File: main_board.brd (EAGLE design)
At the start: 123.2 x 81 mm, 46 parts, among them P1 ST-TF-003A, U1 STM32F407VGT6, U2 USBLC6-2, U3 MCP1700T-3302E, U4 LTC4054LES5-4.2#TRPBF, X1 MicroUSB-B

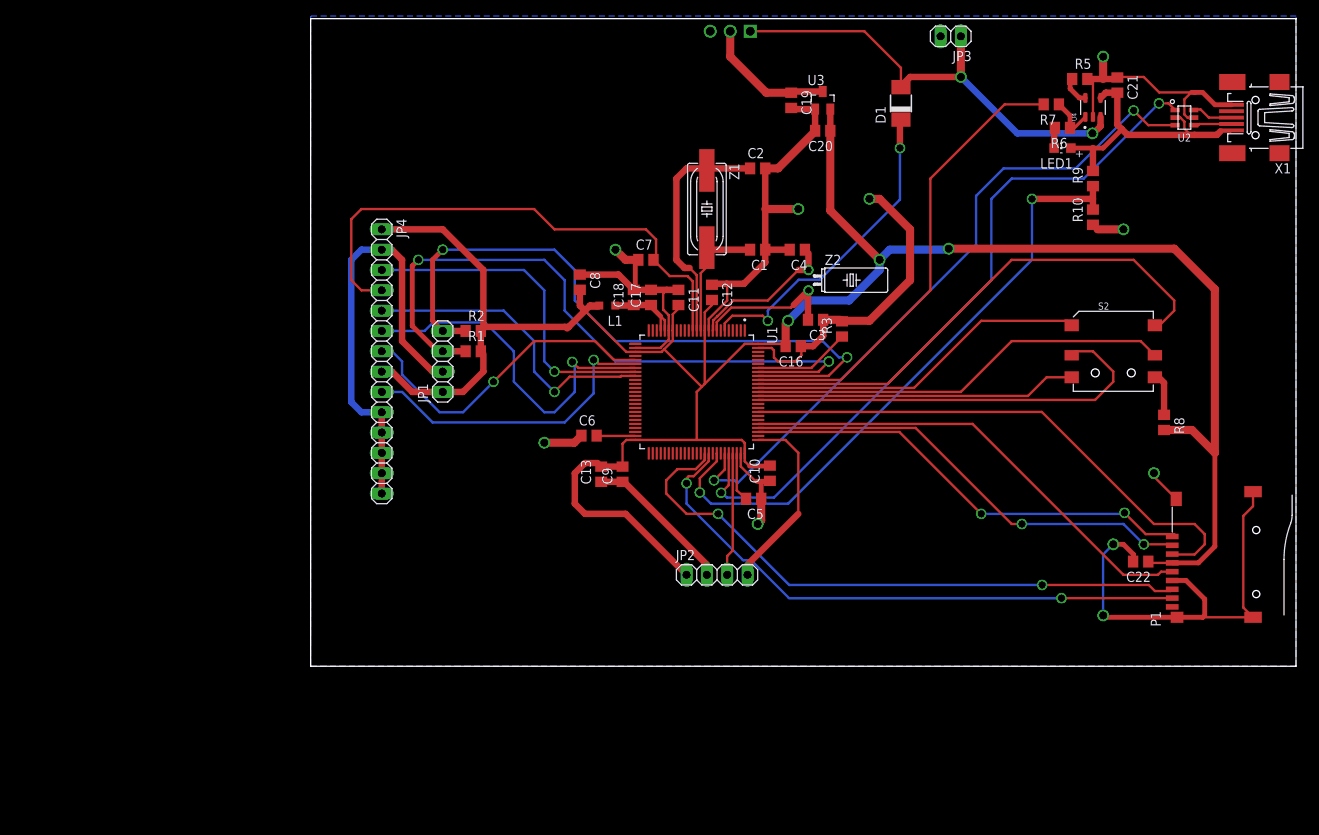
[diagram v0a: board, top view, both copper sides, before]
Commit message: pcb almost done
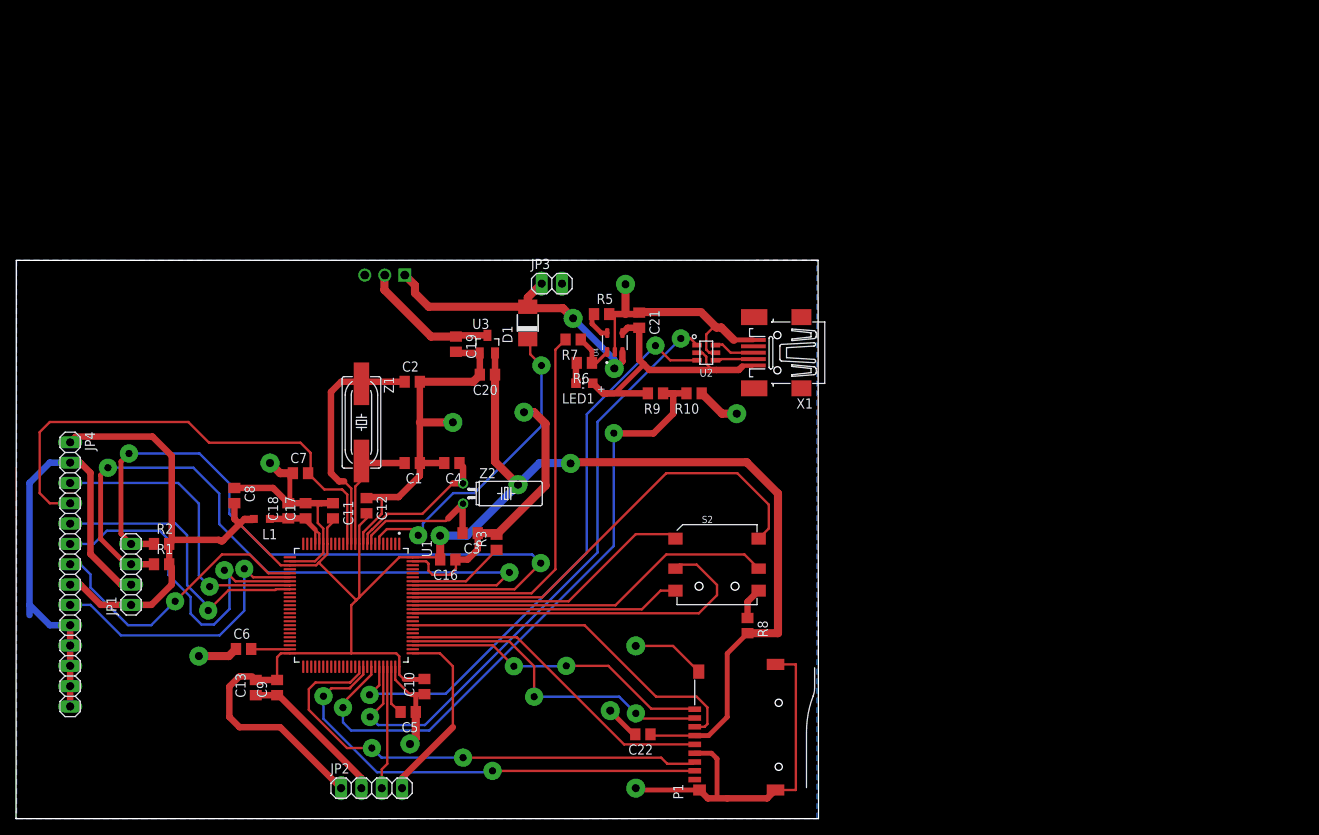
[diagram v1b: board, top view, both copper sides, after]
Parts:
- moved C21 66.6 mm to (77.9, 62.3)
- moved R5 66.6 mm to (73.2, 63.1)
- moved R7 66.6 mm to (69.6, 59.9)
- moved U2 66.6 mm to (86.3, 58.2)
- moved U4 66.6 mm to (74.9, 59.5)
- moved LED1 66.6 mm to (71.0, 54.4)
- moved R6 66.6 mm to (71.0, 57.0)
- moved X1 66.6 mm to (95.2, 58.2)
- moved C22 65.9 mm to (78.4, 10.5)
- moved P1 63.5 mm to (90.2, 10.2)
- moved R9 60.9 mm to (79.9, 53.2), turned to 180 degrees
- moved JP3 58.7 mm to (67.0, 66.9), turned to 0 degrees
- moved R8 57.9 mm to (91.4, 24.1)
- moved S2 56.3 mm to (87.6, 31.8)
- moved R10 54.5 mm to (84.8, 53.2), turned to 180 degrees
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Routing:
- net VDD: track 305.1 -> 281.8 mm
- net SD_CMD: track 68.0 -> 45.1 mm
- net SD_DAT2: track 57.8 -> 38.7 mm
- net SD_CLK: track 59.7 -> 40.8 mm
- net VBAT+: track 58.3 -> 39.7 mm
- net SD_DAT3: track 57.8 -> 41.5 mm
- net SD_DAT0: track 76.7 -> 61.7 mm
- net SD_DAT1: track 73.6 -> 59.2 mm
- net D-_INT: track 85.4 -> 73.9 mm
- net D+_PROT: track 89.0 -> 78.2 mm
- net NCHRG: track 58.1 -> 48.3 mm
- net BTN_0: track 65.0 -> 57.3 mm
- net I2C_SCL: track 84.5 -> 91.8 mm
- net BTN_2: track 53.0 -> 46.6 mm
- net BTN_4: track 53.1 -> 46.7 mm
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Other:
- board size 123.2 x 81 mm -> 100.3 x 69.8 mm
